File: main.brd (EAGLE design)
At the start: 24.4 x 26.2 mm, 45 parts, among them IC1 ATTINY13A-SSH, IC2 TP4056-42-ESOP8, IC3 LM27313XMFX_NOPB, IC4 TPL5110DDCT, IC5 ATTINY13A-SSH, T1A 2N4401, T1B NPN, X1 MINI-USB-UX60A-MB-5ST, X2 332-02

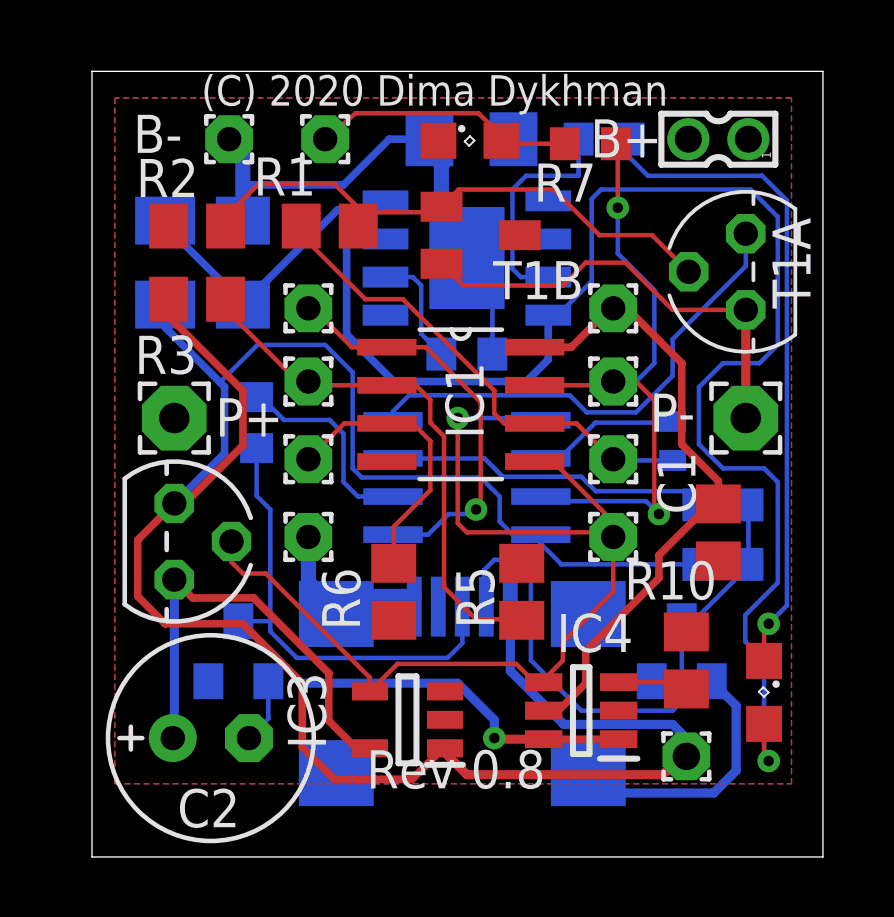
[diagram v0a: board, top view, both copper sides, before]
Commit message: updates
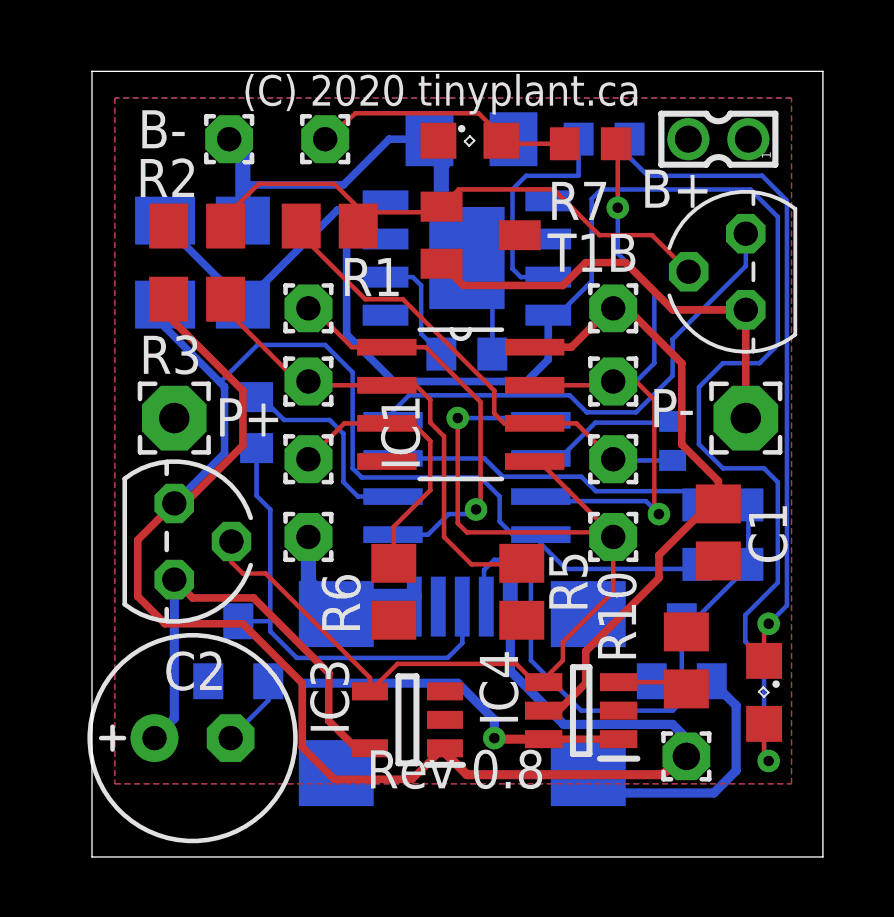
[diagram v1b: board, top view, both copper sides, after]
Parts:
- moved C2 0.61 mm to (4.27, 3.05)
- turned R5 to 270 degrees
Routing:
- net SENSOR+: track 17.9 -> 16.2 mm
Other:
- board text added: "(C) 2020 tinyplant.ca"
- board text removed: "(C) 2020 Dima Dykhman"

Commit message: updates
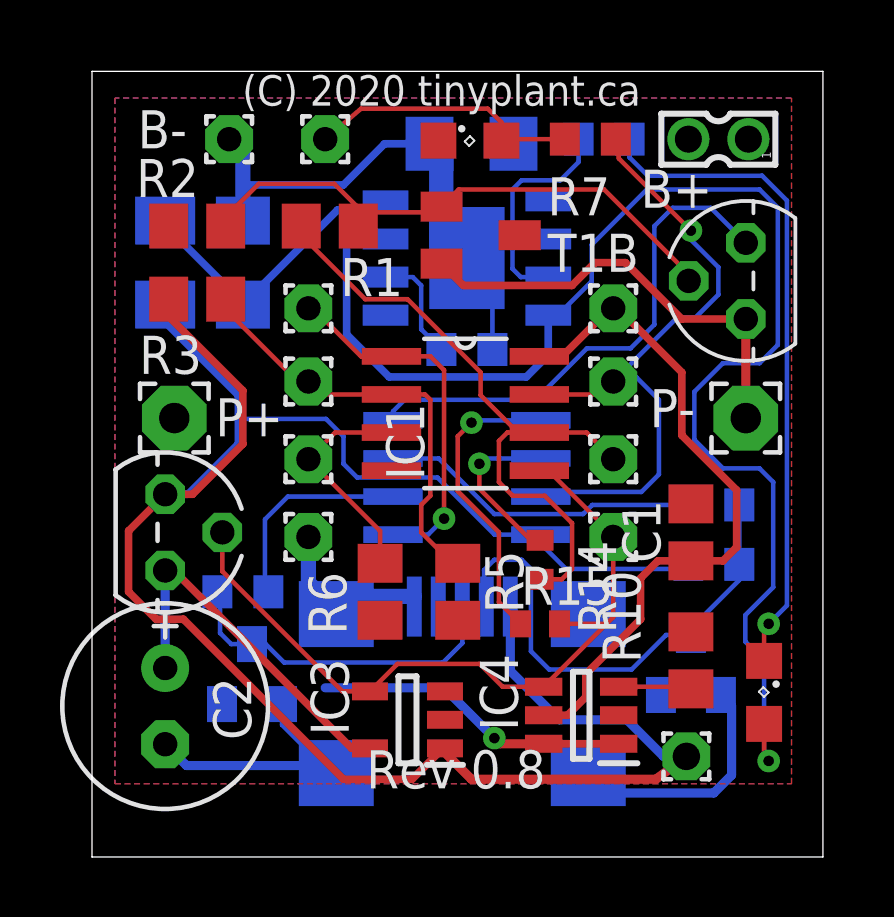
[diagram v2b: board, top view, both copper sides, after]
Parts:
- added R15: 0R, resistor:R0402
- moved R14 5.94 mm to (15.8, 8.99), flipped to the top
- moved R12 5.66 mm to (5.94, 7.92), turned to 180 degrees
- moved R5 2.13 mm to (13.1, 7.92)
- moved C2 1.41 mm to (3.35, 4.11), turned to 270 degrees
- moved C1 0.91 mm to (20.9, 9.91), turned to 270 degrees
- moved D2 0.89 mm to (6.25, 5.18)
- moved D1 0.55 mm to (20.9, 5.49)
- moved R6 0.46 mm to (10.5, 7.92)
- moved REG1A 0.43 mm to (3.35, 9.91)
- moved IC1 0.34 mm to (13.4, 13.9)
- moved R11 0.30 mm to (21.6, 10.8)
- moved R13 0.30 mm to (21.6, 8.84)
- moved T1A 0.30 mm to (22.7, 18.3)
- moved C4 0.15 mm to (13.6, 22.9)
- moved IC4 0.15 mm to (17.2, 3.81)
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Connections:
- new net N$16: IC5.5, R15.1
- net SOLAR_REG+/-: now also R15.2; no longer IC5.5
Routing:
- net N$16: track 0.00 -> 10.1 mm, vias 0 -> 1
- net SOLAR_REG+/-: track 34.7 -> 25.3 mm, vias 1 -> 0
- net NPN+: track 16.2 -> 22.8 mm
- net GND: track 53.3 -> 59.4 mm
- net N$5: track 75.6 -> 71.1 mm
- net N$14: track 15.6 -> 11.4 mm
- net SOLAR_PANEL+: track 15.3 -> 12.5 mm
- net N$13: track 19.7 -> 16.9 mm
- net SENSOR-: track 9.38 -> 7.60 mm
- net N$3: track 21.1 -> 22.9 mm
- net SENSOR+: track 16.2 -> 14.6 mm
- net RESET: track 13.8 -> 12.2 mm
- net VCC: track 11.7 -> 10.6 mm
- net N$4: track 58.6 -> 57.6 mm
- net N$15: track 4.91 -> 5.69 mm, vias 0 -> 1
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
